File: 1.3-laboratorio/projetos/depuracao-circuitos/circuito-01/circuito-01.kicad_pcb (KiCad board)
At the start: 2 copper layers, 49.5 x 48.3 mm, 11 parts, among them P1 CONN_01X02, SW1 SW_DIP_x04, U1 74LS32, U2 7400, U3 74LS386

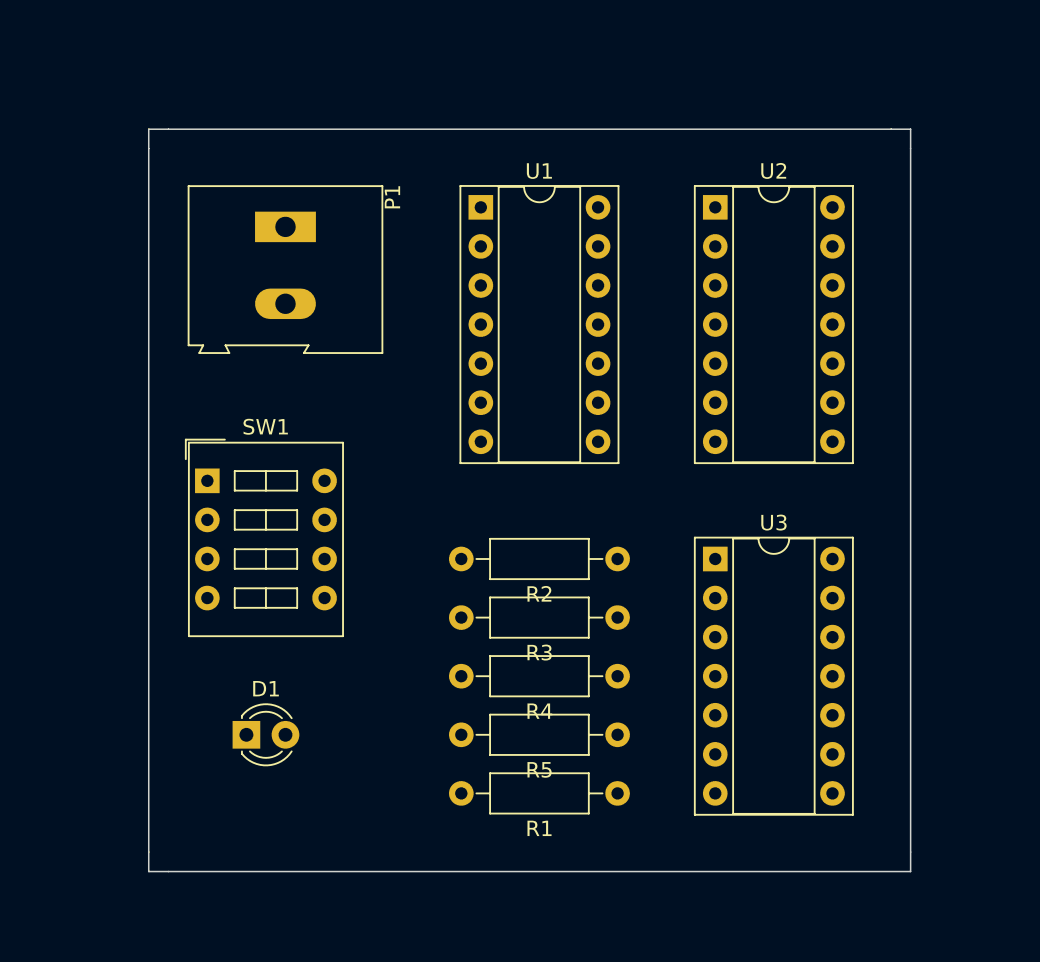
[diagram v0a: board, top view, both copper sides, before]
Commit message: Atualização PCB
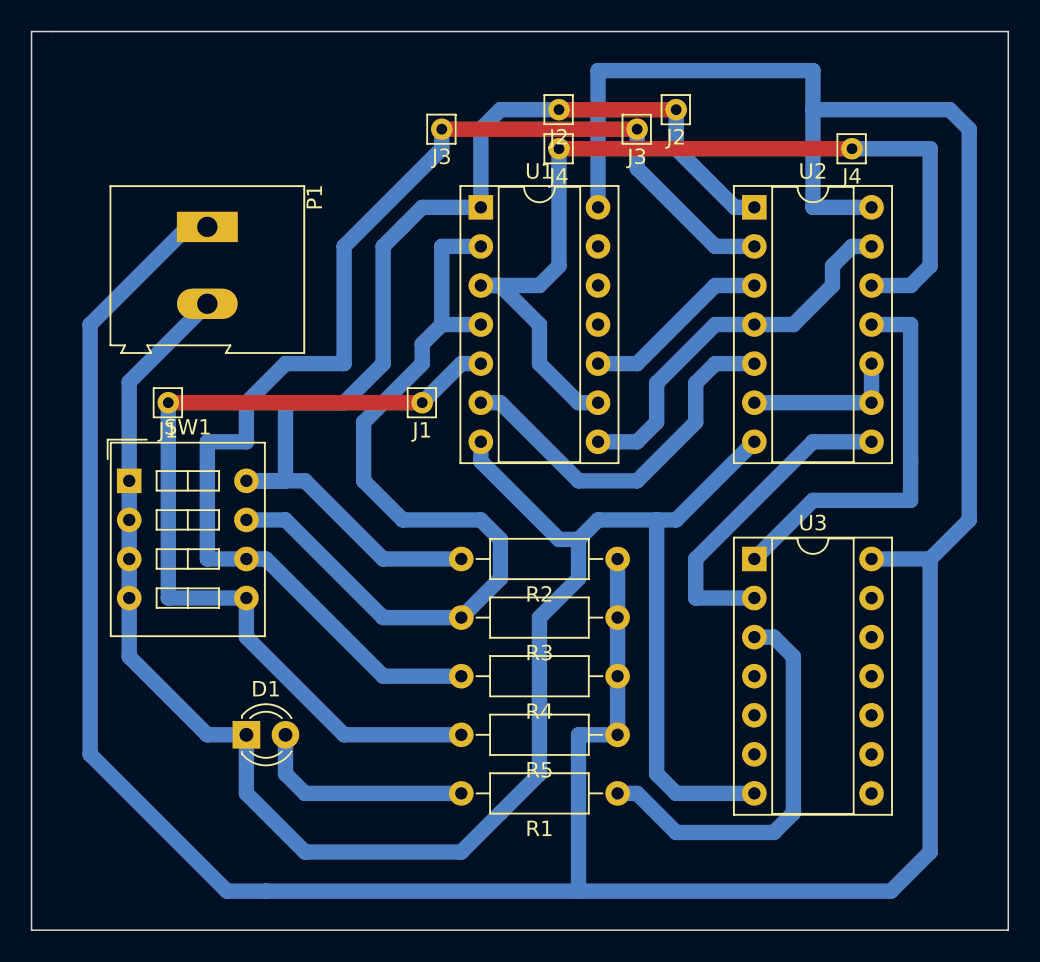
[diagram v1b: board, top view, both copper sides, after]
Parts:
- added J1: J1, Connectors:Pin_d0.7mm_L6.5mm_W1.8mm_FlatFork, F.Cu at (81.3, 61.0)
- added J1: J1, Connectors:Pin_d0.7mm_L6.5mm_W1.8mm_FlatFork, F.Cu at (97.8, 61.0)
- added J2: J2, Connectors:Pin_d0.7mm_L6.5mm_W1.8mm_FlatFork, F.Cu at (106.7, 41.9)
- added J2: J2, Connectors:Pin_d0.7mm_L6.5mm_W1.8mm_FlatFork, F.Cu at (114.3, 41.9)
- added J3: J3, Connectors:Pin_d0.7mm_L6.5mm_W1.8mm_FlatFork, F.Cu at (99.1, 43.2)
- added J3: J3, Connectors:Pin_d0.7mm_L6.5mm_W1.8mm_FlatFork, F.Cu at (111.8, 43.2)
- added J4: J4, Connectors:Pin_d0.7mm_L6.5mm_W1.8mm_FlatFork, F.Cu at (125.7, 44.5)
- added J4: J4, Connectors:Pin_d0.7mm_L6.5mm_W1.8mm_FlatFork, F.Cu at (106.7, 44.5)
- moved P1 5.08 mm to (83.8, 49.5)
- moved SW1 5.08 mm to (78.7, 66.0)
- moved U2 2.54 mm to (119.4, 48.3)
- moved U3 2.54 mm to (119.4, 71.1)
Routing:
- net VCC: track 0.00 -> 219.8 mm
- net GND: track 0.00 -> 124.8 mm
- net Net-(R4-Pad2): track 0.00 -> 69.9 mm
- net Net-(R2-Pad2): track 0.00 -> 66.0 mm
- net (no net): track 0.00 -> 55.9 mm
- net Net-(R3-Pad2): track 0.00 -> 55.6 mm
- net Net-(U1-Pad3): track 0.00 -> 42.5 mm
- net Net-(R5-Pad2): track 0.00 -> 41.8 mm
- net Net-(R1-Pad1): track 0.00 -> 26.2 mm
- net Net-(U2-Pad11): track 0.00 -> 25.7 mm
- net Net-(U1-Pad8): track 0.00 -> 25.3 mm
- net Net-(U1-Pad6): track 0.00 -> 24.5 mm
- net Net-(U2-Pad8): track 0.00 -> 20.9 mm
- net Net-(D1-Pad2): track 0.00 -> 14.5 mm
- net Net-(U1-Pad10): track 0.00 -> 12.3 mm
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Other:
- board size 49.5 x 48.3 mm -> 63.5 x 58.4 mm
- net class Alimentacao: clearance 1 -> 0.5; trace_width 1.5 -> 1
